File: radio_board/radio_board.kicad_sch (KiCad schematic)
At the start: 82 parts, among them CN1 HX JN1.27-2X5P ZZ H4.9, Q1 2N7002K, SW2 RKB2SJG250SMTRLFS, SW3 MSK12C02, U1 FSC-BT1036C, U2 TP4057, U3 XB5352A, U4 SKB369, U5 S2B-PH-K-S(LF)(SN), U6 TLV75533PDBVR, U7 LMV321

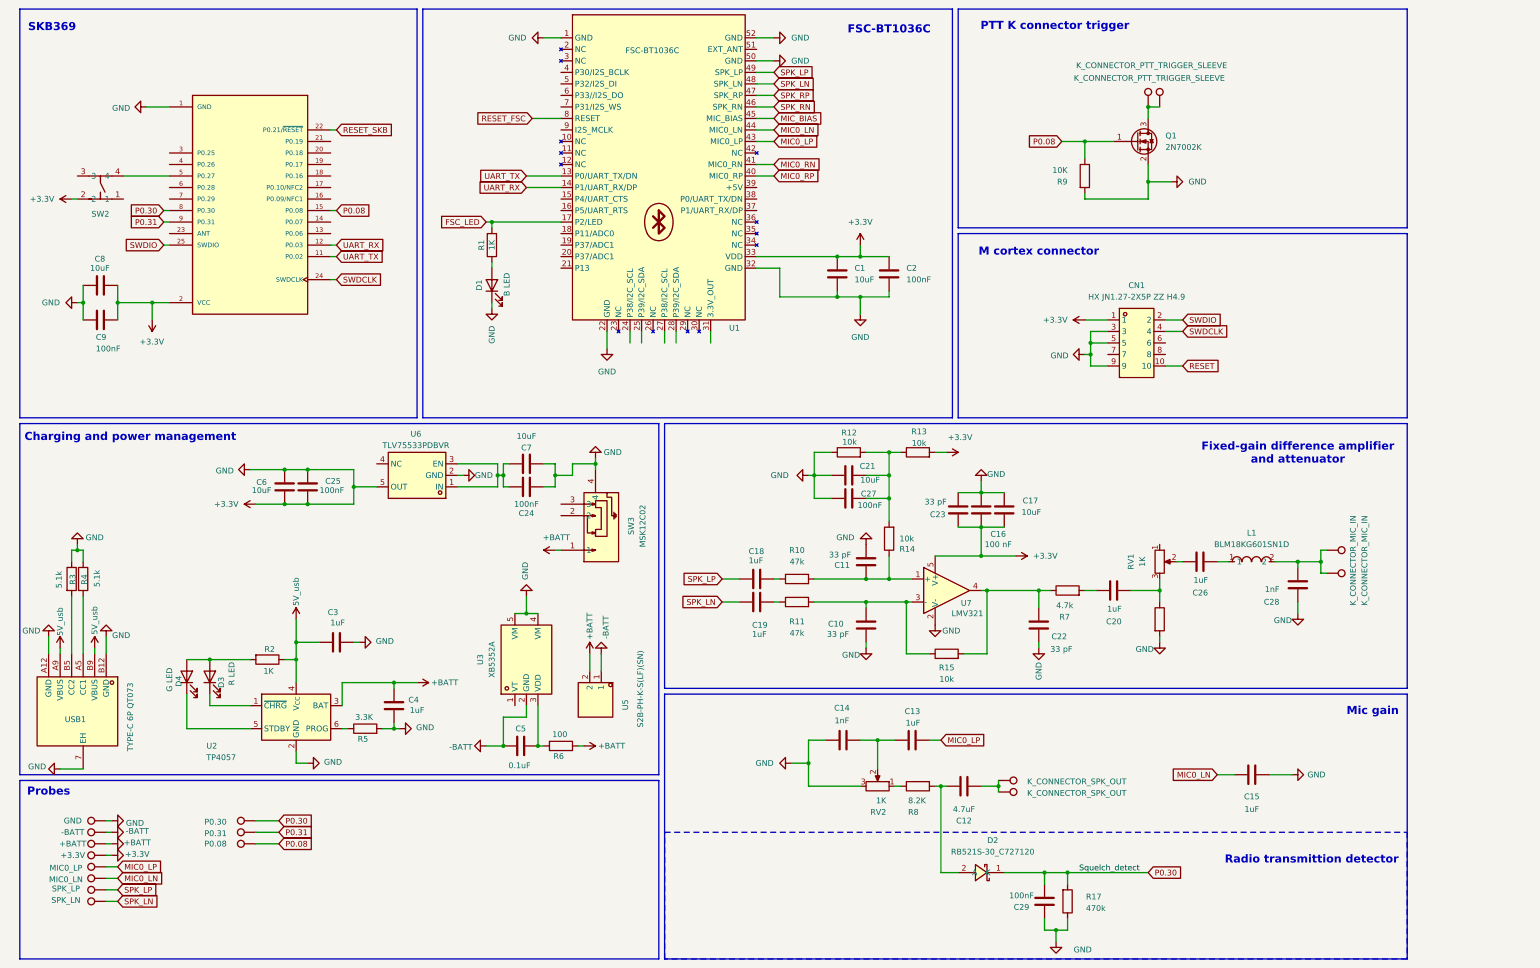
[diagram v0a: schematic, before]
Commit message: [WIP]
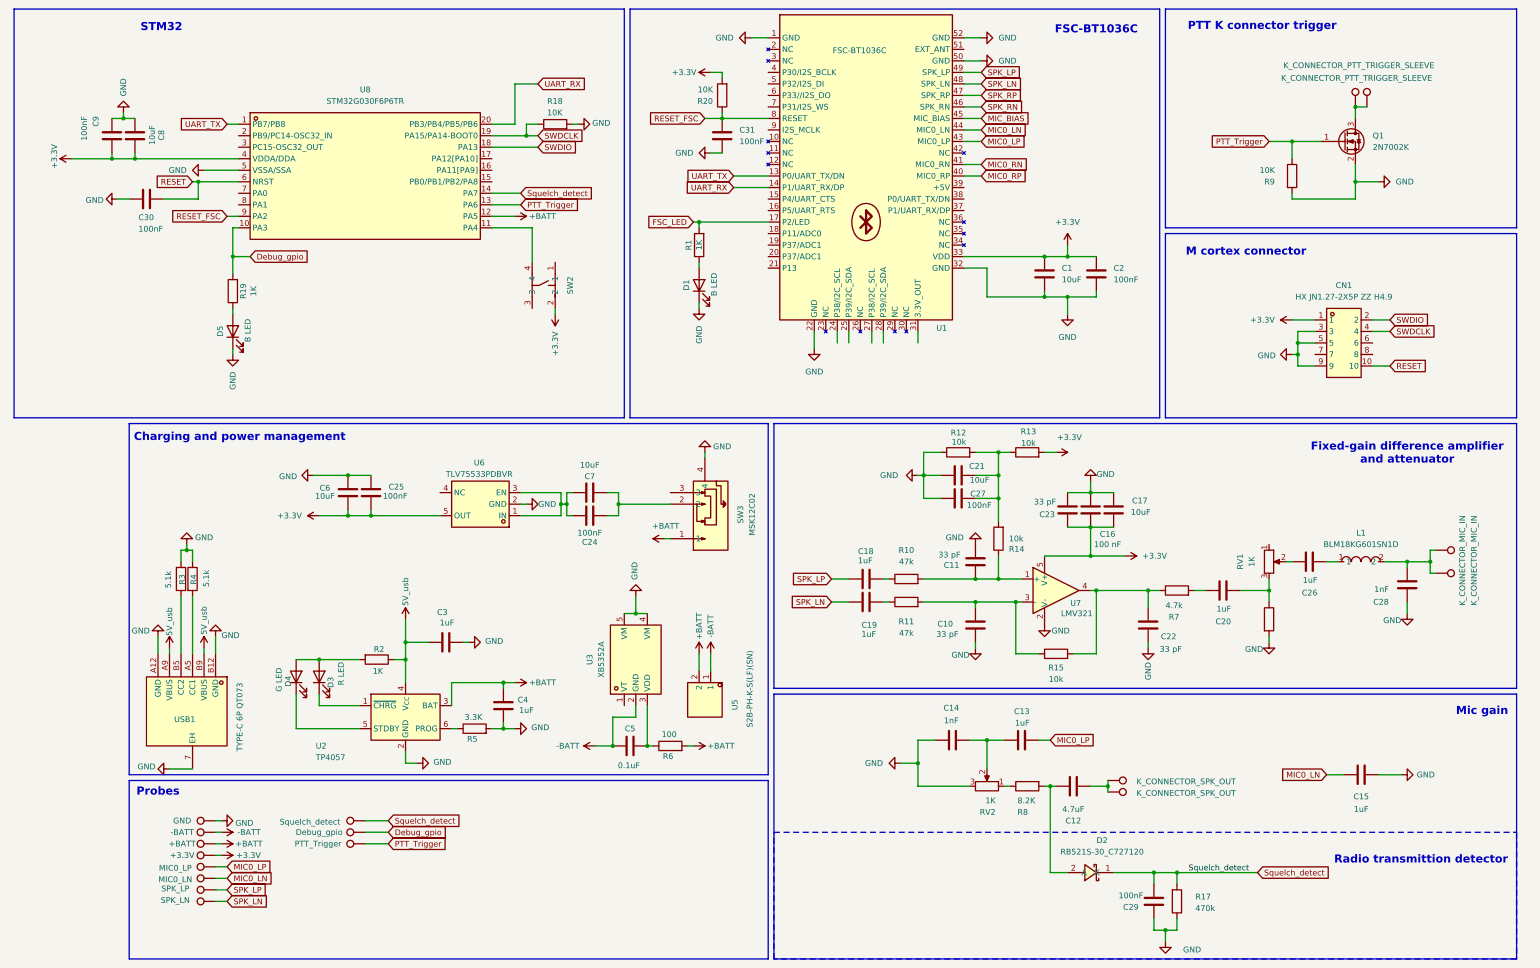
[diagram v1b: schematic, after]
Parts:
- removed U4: SKB369, PTT_Project_library:SKYLAB_SKB369, symbol PTT_Project_library:SKB369
- added C30, C31: 100nF, Resistor_SMD:R_0603_1608Metric_Pad0.98x0.95mm_HandSolder, symbol Device:C
- added D5: B LED, LED_SMD:LED_0603_1608Metric_Pad1.05x0.95mm_HandSolder, symbol Device:LED
- added R18, R20: 10K, Resistor_SMD:R_0603_1608Metric_Pad0.98x0.95mm_HandSolder, symbol Device:R
- added R19: 1K, Resistor_SMD:R_0603_1608Metric_Pad0.98x0.95mm_HandSolder, symbol Device:R
- added U8: STM32G030F6P6TR, PTT_Project_library:TSSOP-20_L6.5-W4.4-P0.65-LS6.4-BL, symbol PTT_Project_library:STM32G030F6P6TR
- TP2: value P0.08 -> PTT_Trigger
- TP44: value P0.30 -> Squelch_detect
- TP52: value P0.31 -> Debug_gpio
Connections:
- net +3.3V: now also R20.2, U8.4 (VDDA/DDA); no longer C1.1, C10.2, C11.2, C14.1, C15.1, C16.1, C17.1, C2.1, C21.1, C22.1, C23.1, C24.1, C25.1, C27.1, C28.2, C29.2, C3.1, C4.2, C6.1, C7.1, C8.1, C9.1, CN1.3, CN1.5, CN1.9, D1.1 (K), Q1.2 (S), R12.1, R16.2, R17.1, R3.1, R4.1, R5.2, R9.2, RV2.3, SW3.4, TP5.1, U1.1 (GND), U1.22 (GND), U1.32 (GND), U1.50 (GND), U1.52 (GND), U2.2 (GND), U3.4 (VM), U3.5 (VM), U6.2 (GND), U7.2 (V-), USB1.7 (EH), USB1.A12 (GND), USB1.B12 (GND)
- net +BATT: now also U8.12 (PA5)
- net RESET: now also C30.1, U8.6 (NRST)
- net RESET_FSC: now also C31.2, R20.1, U8.9 (PA2)
- net SWDCLK: now also R18.1, U8.19 (PA15/PA14-BOOT0)
- net SWDIO: now also U8.18 (PA13)
- net UART_RX: now also U8.20 (PB3/PB4/PB5/PB6)
- net UART_TX: now also U8.1 (PB7/PB8)
- net at SW2.4: now also U8.11 (PA4)
- net at SW3.2: now also C24.1, C7.1
- net P0.08 renamed PTT_Trigger
- net PTT_Trigger: now also U8.13 (PA6)
- net P0.30 renamed Squelch_detect
- net Squelch_detect: now also U8.14 (PA7)
- net P0.31 renamed Debug_gpio
- net Debug_gpio: now also R19.2, U8.10 (PA3)
- new net: D5.2 (A), R19.1
- new net GND: C1.1, C10.2, C11.2, C14.1, C15.1, C16.1, C17.1, C2.1, C21.1, C22.1, C23.1, C25.1, C27.1, C28.2, C29.2, C3.1, C30.2, C31.1, C4.2, C6.1, C8.1, C9.1, CN1.3, CN1.5, CN1.9, D1.1 (K), D5.1 (K), Q1.2 (S), R12.1, R16.2, R17.1, R18.2, R3.1, R4.1, R5.2, R9.2, RV2.3, SW3.4, TP5.1, U1.1 (GND), U1.22 (GND), U1.32 (GND), U1.50 (GND), U1.52 (GND), U2.2 (GND), U3.4 (VM), U3.5 (VM), U6.2 (GND), U7.2 (V-), U8.5 (VSSA/SSA), USB1.7 (EH), USB1.A12 (GND), USB1.B12 (GND)
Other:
- note added: "STM32"
- note removed: "SKB369"
- moved on the sheet: C1, C10, C11, C12, C13, C14, C15, C16, C17, C18, C19, C2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

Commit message: [WIP]
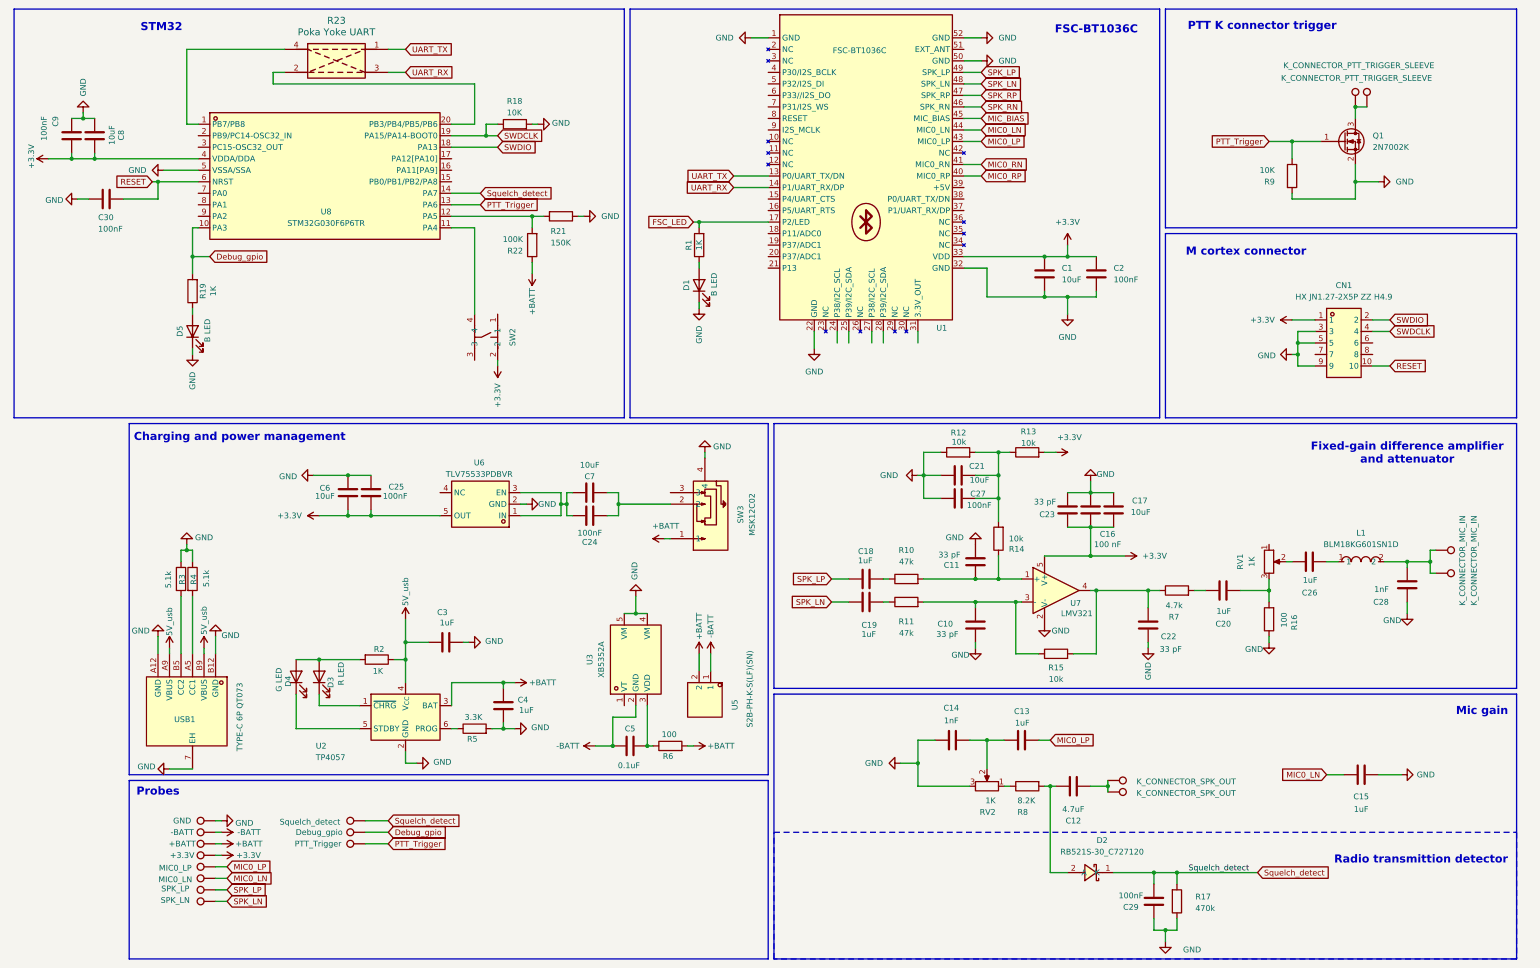
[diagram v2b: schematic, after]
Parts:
- removed C31: 100nF, Resistor_SMD:R_0603_1608Metric_Pad0.98x0.95mm_HandSolder, symbol Device:C
- removed R20: 10K, Resistor_SMD:R_0603_1608Metric_Pad0.98x0.95mm_HandSolder, symbol Device:R
- added R21: 150K, Resistor_SMD:R_0603_1608Metric_Pad0.98x0.95mm_HandSolder, symbol Device:R
- added R22: 100K, Resistor_SMD:R_0603_1608Metric_Pad0.98x0.95mm_HandSolder, symbol Device:R
- added R23: Poka Yoke UART, poka_yuke:poka_yoke_uart_Solder, symbol poka_yoke:Poka Yoke UART
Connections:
- net +BATT: now also R22.1; no longer U8.12 (PA5)
- net GND: now also R16.1, R21.1; no longer R16.2
- net UART_RX: now also R23.3; no longer U8.20 (PB3/PB4/PB5/PB6)
- net UART_TX: now also R23.1; no longer U8.1 (PB7/PB8)
- net at C20.2, RV1.3: now also R16.2; no longer R16.1
- net RESET_FSC: no longer names the net of U8.9 (PA2)
- net RESET_FSC: no longer U1.8 (RESET)
- new net: R23.4, U8.1 (PB7/PB8)
- new net: R21.2, R22.2, U8.12 (PA5)
- new net: R23.2, U8.20 (PB3/PB4/PB5/PB6)
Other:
- moved on the sheet: C30, C8, C9, D5, R18, R19, SW2, U8

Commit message: [WIP]
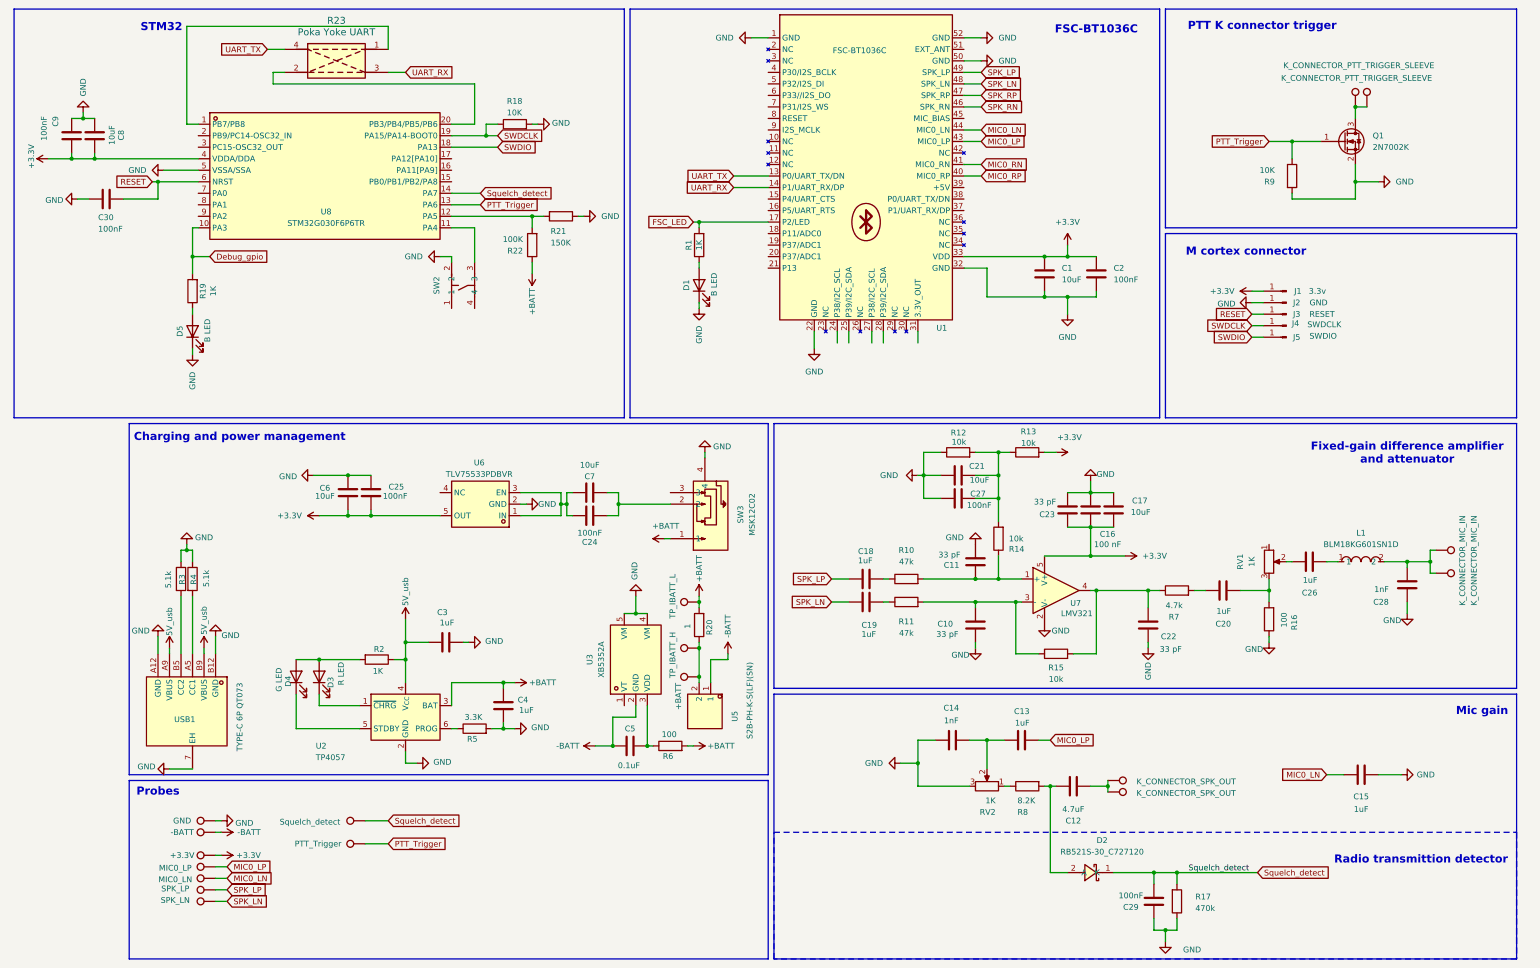
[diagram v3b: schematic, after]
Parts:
- removed CN1: HX JN1.27-2X5P ZZ H4.9, PTT_Project_library:CONN-TH_10P-P1.27_HX-JN1.27-2X5P-ZZ-H4.9, symbol PTT_Project_library:HXJN1.27-2X5PZZH4.9
- removed TP52: Debug_gpio, TestPoint:TestPoint_THTPad_D2.0mm_Drill1.0mm, symbol Connector:TestPoint
- added J1: 3.3v, Connector_PinSocket_2.54mm:PinSocket_1x01_P2.54mm_Vertical, symbol Connector:Conn_01x01_Pin
- added J2: GND, Connector_PinSocket_2.54mm:PinSocket_1x01_P2.54mm_Vertical, symbol Connector:Conn_01x01_Pin
- added J3: RESET, Connector_PinSocket_2.54mm:PinSocket_1x01_P2.54mm_Vertical, symbol Connector:Conn_01x01_Pin
- added J4: SWDCLK, Connector_PinSocket_2.54mm:PinSocket_1x01_P2.54mm_Vertical, symbol Connector:Conn_01x01_Pin
- added J5: SWDIO, Connector_PinSocket_2.54mm:PinSocket_1x01_P2.54mm_Vertical, symbol Connector:Conn_01x01_Pin
- added R20: 1, Resistor_SMD:R_0603_1608Metric_Pad0.98x0.95mm_HandSolder, symbol Device:R
- added TP1: TP_IBATT_H, TestPoint:TestPoint_THTPad_D2.0mm_Drill1.0mm, symbol Connector:TestPoint
- added TP3: TP_IBATT_L, TestPoint:TestPoint_THTPad_D2.0mm_Drill1.0mm, symbol Connector:TestPoint
- TP47: footprint TestPoint:TestPoint_Pad_D3.0mm -> TestPoint:TestPoint_Pad_D2.5mm
- TP6: footprint TestPoint:TestPoint_THTPad_D2.0mm_Drill1.0mm -> TestPoint:TestPoint_Pad_D2.5mm
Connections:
- net +3.3V: now also J1.1 (Pin_1); no longer SW2.2
- net +BATT: now also R20.2, TP3.1; no longer TP47.1, U5.2
- net GND: now also SW2.2, J2.1 (Pin_1)
- net RESET: now also J3.1 (Pin_1)
- net SWDCLK: now also J4.1 (Pin_1)
- net SWDIO: now also J5.1 (Pin_1)
- net UART_TX: now also R23.4; no longer R23.1
- net at U8.1 (PB7/PB8): now also R23.1; no longer R23.4
- net at U8.11 (PA4): now also SW2.3; no longer SW2.4
- net MIC_BIAS: no longer names the net of U1.45 (MIC_BIAS)
- new net: R20.1, TP1.1, TP47.1, U5.2
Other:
- moved on the sheet: SW2, U5
